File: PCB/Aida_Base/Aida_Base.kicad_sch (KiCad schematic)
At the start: 106 parts, among them J1 AudioJack4, J10 Conn_01x04_Pin, J2 USB_C_Receptacle_L, J3 Conn_01x02_Pin, J4 Conn_01x03_Pin, J5 Conn_01x04_Pin, J6 Conn_01x04_Pin, J7 Conn_01x02_Pin, J8 Conn_02x02_Odd_Even, J9 Conn_01x03_Pin, Q1 BSS138, SW1 BOOT, SW2 RESET, U1 NCP1117-3.3_SOT223, U2 RP2040_L, U3 W25Q128JVS, Y1 12MHz

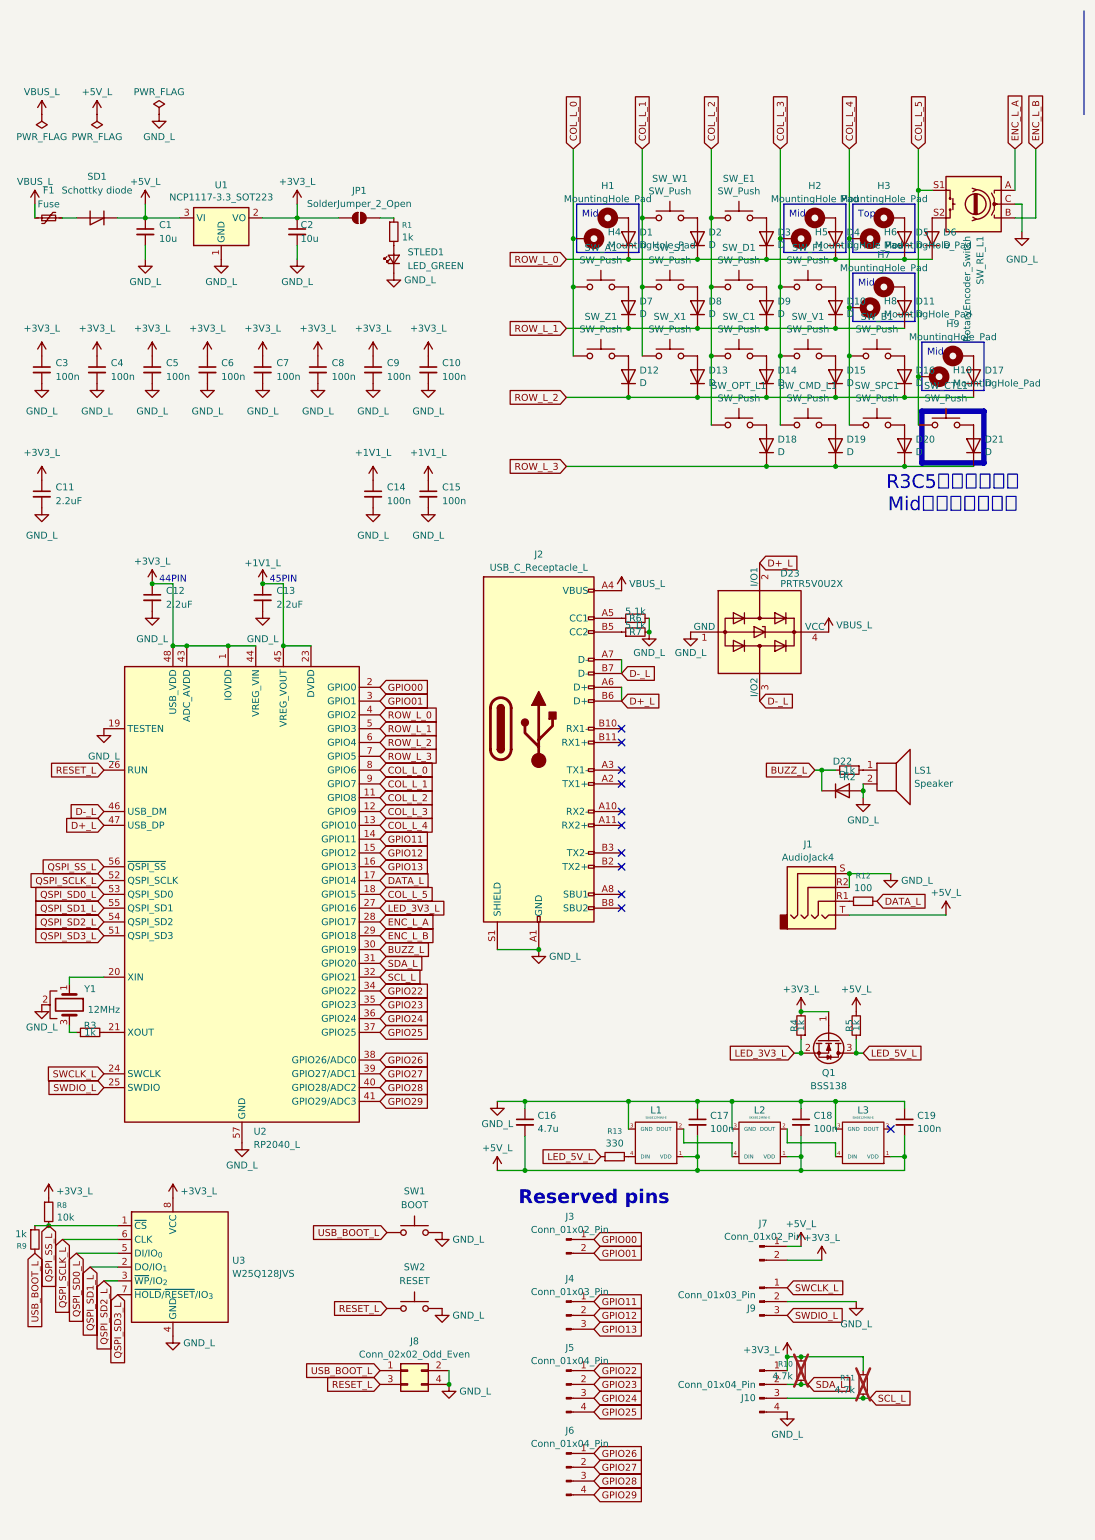
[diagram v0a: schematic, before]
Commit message: 左手の回路が完成
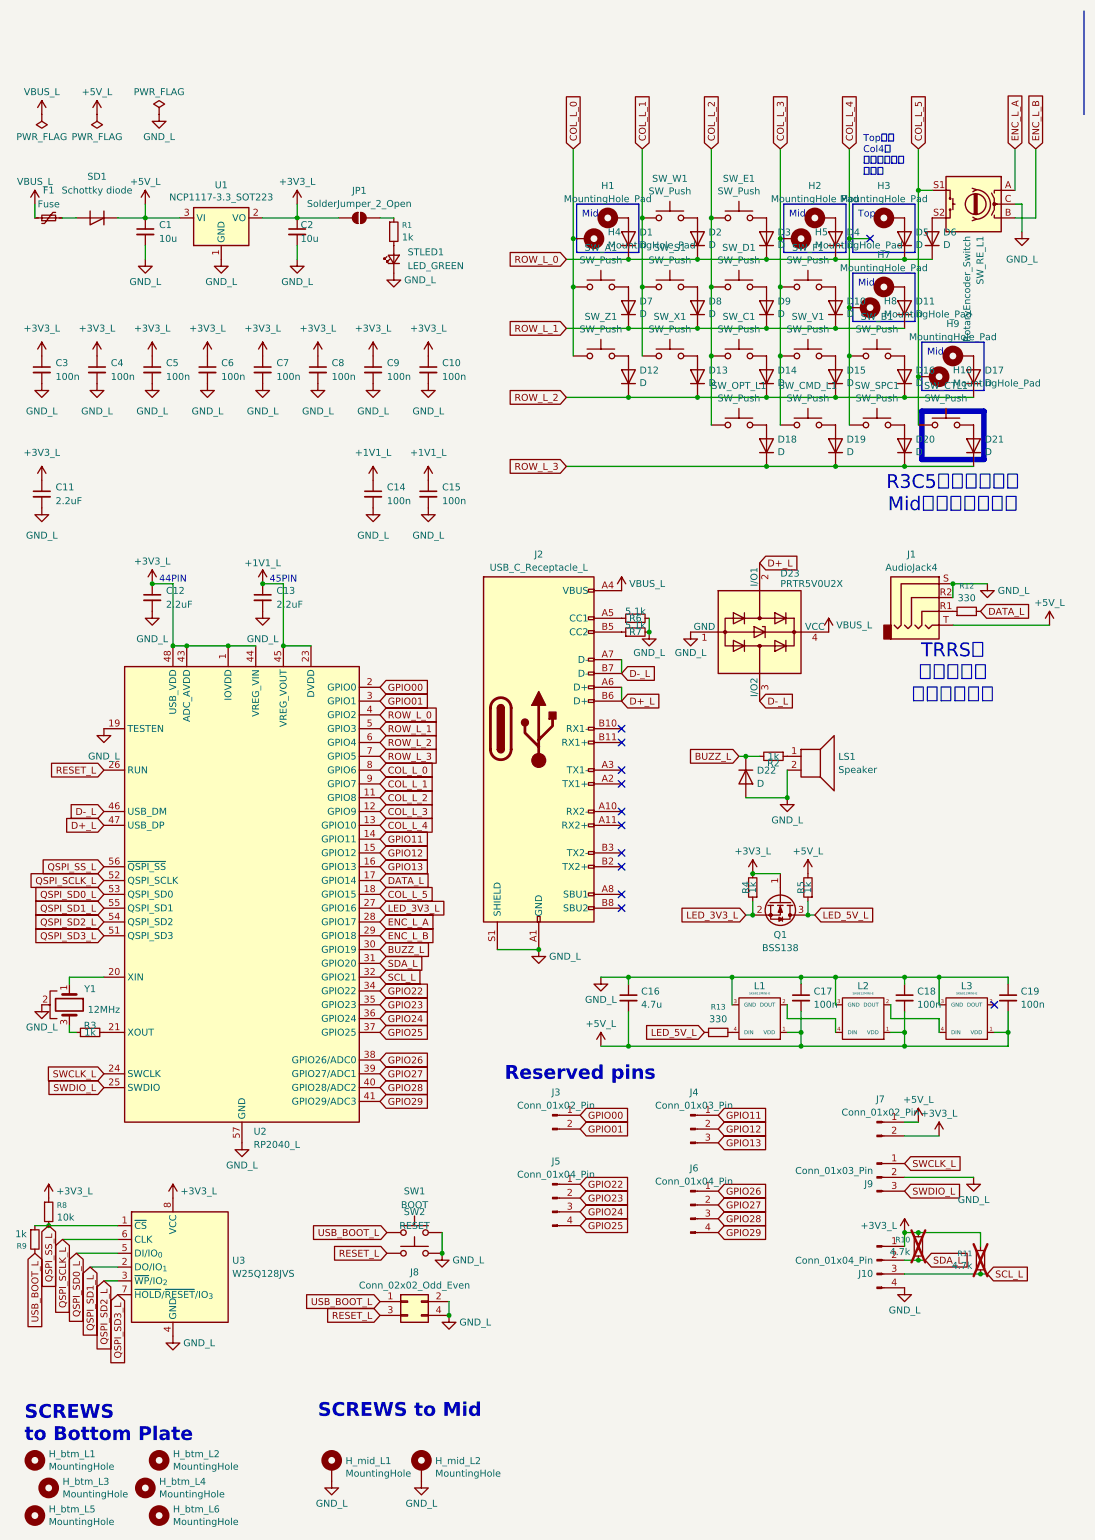
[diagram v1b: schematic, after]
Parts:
- removed H6: MountingHole_Pad, symbol Mechanical:MountingHole_Pad
- added H_btm_L1, H_btm_L2, H_btm_L3, H_btm_L4, H_btm_L5, H_btm_L6: MountingHole, Lib_Local:MountingHole_2.2mm_M2_No_Cu, symbol Mechanical:MountingHole
- added H_mid_L1, H_mid_L2: MountingHole, Lib_Local:MountingHole_1.8-2.2mm_M2_Pad_minimal, symbol Mechanical:MountingHole_Pad
- R12: value 100 -> 330
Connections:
- net GND_L: now also H_mid_L1.1, H_mid_L2.1
- no-connect marks 11 -> 12
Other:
- note added: "SCREWS to Bottom Plate"
- note added: "SCREWS to Mid"
- note added: "TRRSに 保護回路が あってもよい"
- note added: "Topへの Col4は 下のスイッチ と共通"
- moved on the sheet: C16, C17, C18, C19, D22, J1, J10, J3, J4, J5, J6, J7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
